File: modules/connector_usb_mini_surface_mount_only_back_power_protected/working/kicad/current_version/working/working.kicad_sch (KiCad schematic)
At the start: 2 parts, among them J3 scumnsmo

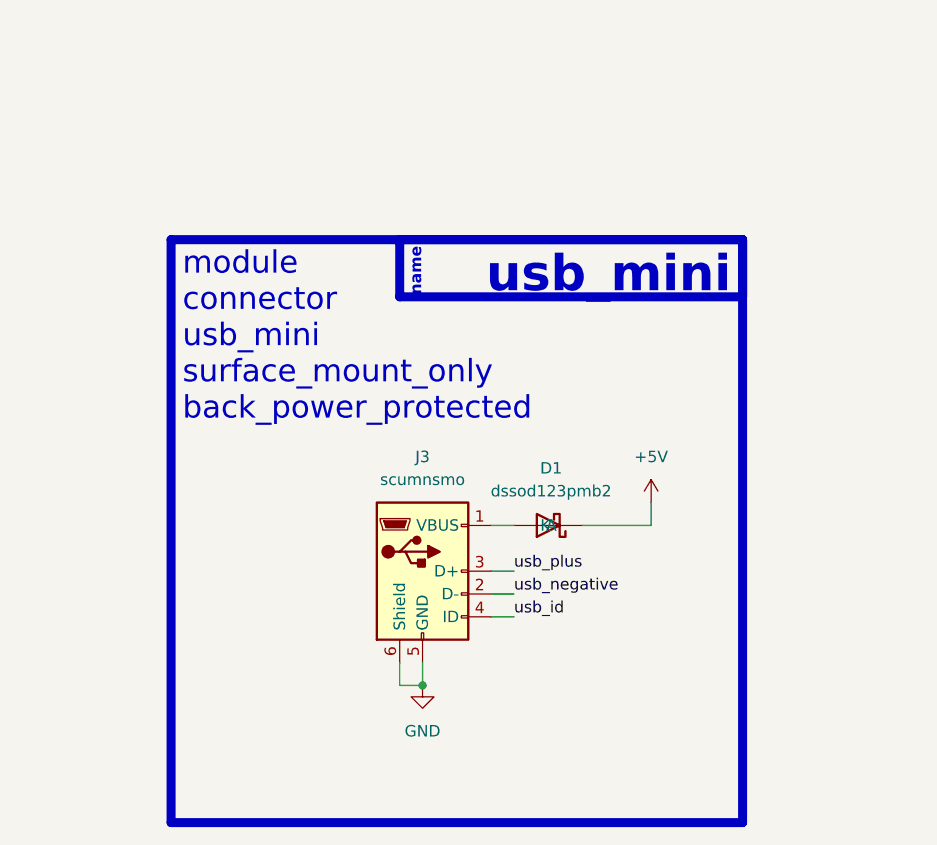
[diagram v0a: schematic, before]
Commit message: a few module workings
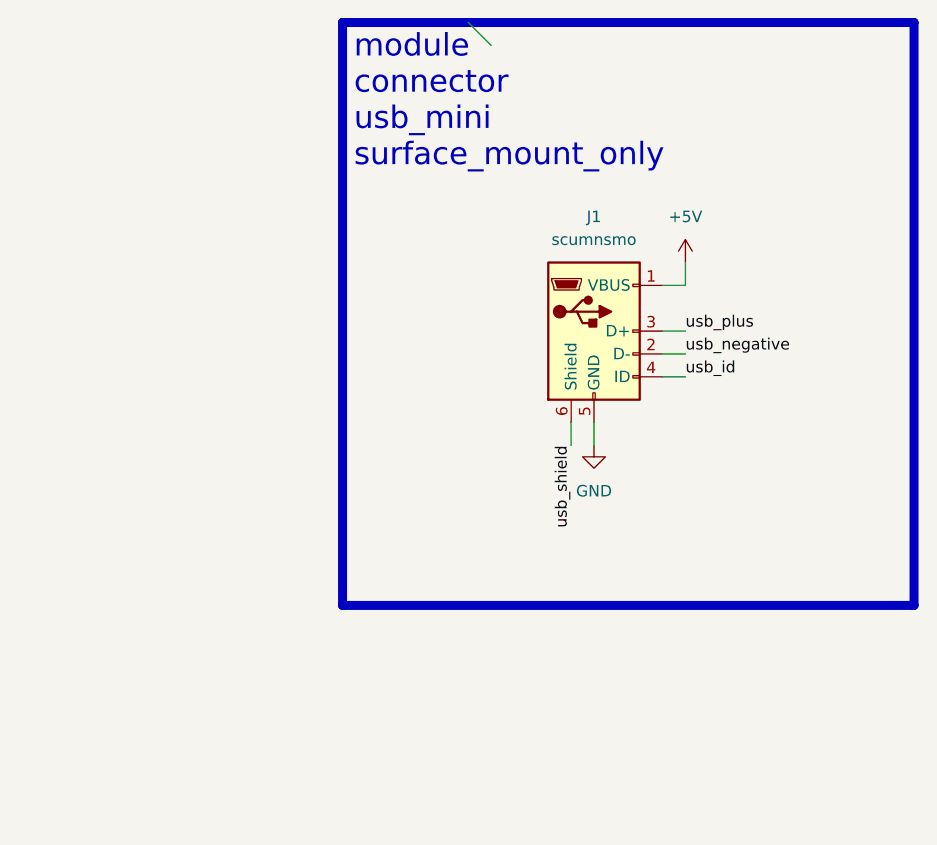
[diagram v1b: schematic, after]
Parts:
- removed D1: dssod123pmb2, oomlout_oomp_part_footprints:dssod123pmb2_electronic_diode_schottky_sod_123_package_marking_b2_mbr0520, symbol oomlout_oomp_part_symbols:dssod123pmb2_electronic_diode_schottky_sod_123_packag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
- removed J3: scumnsmo, oomlout_oomp_part_kicad_footprints:scumnsmo_electronic_socket_usb_mini_surface_mount_only, symbol oomlout_oomp_part_symbols:scumnsmo_electronic_socket_usb_mini_surface_mount_only
- added J1: scumnsmo, scumnsmo_electronic_socket_usb_mini_surface_mount_only, symbol oomlout_oomp_part_symbols:scumnsmo_electronic_socket_usb_mini_surface_mount_only
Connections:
- net +5V: now also J1.1 (VBUS)
- net GND: now also J1.5 (GND)
- net usb_id: now also J1.4 (ID)
- net usb_negative: now also J1.2 (D-)
- net usb_plus: now also J1.3 (D+)
- new net usb_shield: J1.6 (Shield)
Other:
- note added: "module connector usb_mini surface_mount_only"
- note removed: "module connector usb_mini surface_mount_only back_power_protected"
- note removed: "name"
- note removed: "usb_mini"
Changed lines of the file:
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@@
 (kicad_sch (version 20230121) (generator eeschema)
   (paper "A4")
-  (junction (at 146.05 114.3) (diameter 0) (color 0 0 0 0)
-  )
-  (wire (pts (xy 153.67 101.6) (xy 156.21 101.6))
+  (bus_entry (at 151.13 40.64) (size 2.54 2.54)
     (stroke (width 0) (type default))
   )
-  (wire (pts (xy 143.51 114.3) (xy 146.05 114.3))
+  (wire (pts (xy 175.26 69.85) (xy 172.72 69.85))
     (stroke (width 0) (type default))
   )
-  (wire (pts (xy 146.05 111.76) (xy 146.05 114.3))
+  (wire (pts (xy 165.1 85.09) (xy 165.1 87.63))
     (stroke (width 0) (type default))
   )
-  (wire (pts (xy 153.67 96.52) (xy 156.21 96.52))
+  (wire (pts (xy 162.56 85.09) (xy 162.56 87.63))
     (stroke (width 0) (type default))
   )
-  (wire (pts (xy 143.51 111.76) (xy 143.51 114.3))
+  (wire (pts (xy 172.72 74.93) (xy 175.26 74.93))
     (stroke (width 0) (type default))
   )
-  (wire (pts (xy 171.45 96.52) (xy 163.83 96.52))
+  (wire (pts (xy 172.72 80.01) (xy 175.26 80.01))
     (stroke (width 0) (type default))
   )
-  (wire (pts (xy 153.67 104.14) (xy 156.21 104.14))
+  (wire (pts (xy 175.26 67.31) (xy 175.26 69.85))
     (stroke (width 0) (type default))
   )
-  (wire (pts (xy 171.45 93.98) (xy 171.45 96.52))
+  (wire (pts (xy 172.72 77.47) (xy 175.26 77.47))
     (stroke (width 0) (type default))
   )
-  (wire (pts (xy 153.67 106.68) (xy 156.21 106.68))
-    (stroke (width 0) (type default))
-  )
-  (rectangle (start 143.51 64.77) (end 181.61 71.12)
-    (stroke (width 1) (type default))
-    (fill (type color) (color 0 0 0 0))
-  )
-  (rectangle (start 118.11 64.77) (end 181.61 129.54)
+  (rectangle (start 137.16 40.64) (end 200.66 105.41)
     (stroke (width 1) (type default))
     (fill (type none))
   )
-  (text "module\nconnector\nusb_mini\nsurface_mount_only\nback_power_protected\n"
-    (at 119.38 85.09 0)
+  (rectangle (start 199.39 97.79) (end 199.39 97.79)
+    (stroke (width 0) (type default))
+    (fill (type none))
+  )
+  (text "module\nconnector\nusb_mini\nsurface_mount_only\n\n" (at 138.43 60.96 0)
     (effects (font (size 2.5 2.5)) (justify left bottom))
   )
-  (text "usb_mini\n" (at 180.34 71.12 0)
-    (effects (font (size 4 4) (thickness 0.8) bold (color 255 255 255 1)) (justify right bottom))
-  )
-  (text "name" (at 146.05 71.12 90)
-    (effects (font (size 1.27 1.27) (thickness 0.254) bold (color 255 255 255 1)) (justify left bottom))
-  )
-  (label "usb_id" (at 156.21 106.68 0) (fields_autoplaced)
+  (label "usb_id" (at 175.26 80.01 0) (fields_autoplaced)
     (effects (font (size 1.27 1.27)) (justify left bottom))
   )
-  (label "usb_negative" (at 156.21 104.14 0) (fields_autoplaced)
+  (label "usb_plus" (at 175.26 74.93 0) (fields_autoplaced)
     (effects (font (size 1.27 1.27)) (justify left bottom))
   )
-  (label "usb_plus" (at 156.21 101.6 0) (fields_autoplaced)
+  (label "usb_negative" (at 175.26 77.47 0) (fields_autoplaced)
     (effects (font (size 1.27 1.27)) (justify left bottom))
   )
-  (symbol (lib_id "oomlout_oomp_part_symbols:scumnsmo_electronic_socket_usb_mini_surface_mount_only") (at 146.05 101.6 0) (unit 1)
+  (label "usb_shield" (at 162.56 87.63 270) (fields_autoplaced)
+    (effects (font (size 1.27 1.27)) (justify right bottom))
+  )
+  (symbol (lib_id "oomlout_oomp_part_symbols:scumnsmo_electronic_socket_usb_mini_surface_mount_only") (at 165.1 74.93 0) (unit 1)
     (in_bom yes) (on_board yes) (dnp no) (fields_autoplaced)
-    (property "Reference" "J3" (at 146.05 88.9 0)
+    (property "Reference" "J1" (at 165.1 62.23 0)
       (effects (font (size 1.27 1.27)))
     )
-    (property "Value" "scumnsmo" (at 146.05 91.44 0)
+    (property "Value" "scumnsmo" (at 165.1 64.77 0)
       (effects (font (size 1.27 1.27)))
     )
-    (property "Footprint" "oomlout_oomp_part_kicad_footprints:scumnsmo_electronic_socket_usb_mini_surface_mount_only" (at 149.86 102.87 0)
+    (property "Footprint" "scumnsmo_electronic_socket_usb_mini_surface_mount_only" (at 168.91 76.2 0)
       (effects (font (size 1.27 1.27)) hide)
     )
-    (property "Datasheet" "https://github.com/oomlout/oomlout_oomp_v3/parts/electronic_socket_usb_mini_surface_mount_only/datasheet.pdf" (at 149.86 102.87 0)
+    (property "Datasheet" "https://github.com/oomlout/oomlout_oomp_v3/parts/electronic_socket_usb_mini_surface_mount_only/datasheet.pdf" (at 168.91 76.2 0)
       (effects (font (size 1.27 1.27)) hide)
     )
@@
     (instances
       (project "working"
-        (path "/5407c114-4107-4d84-8382-1717fb9d687c"
-          (reference "J3") (unit 1)
-        )
-      )
-      (project "working"
         (path "/d7ac9d55-1973-40f4-b2a5-38a433b49fa0"
           (reference "J1") (unit 1)
@@
     )
   )
-  (symbol (lib_id "oomlout_oomp_part_symbols:dssod123pmb2_electronic_diode_schottky_sod_123_package_marking_b2_mbr0520") (at 160.02 96.52 180) (unit 1)
+  (symbol (lib_id "power:+5V") (at 175.26 67.31 0) (unit 1)
     (in_bom yes) (on_board yes) (dnp no) (fields_autoplaced)
-    (property "Reference" "D1" (at 160.3375 90.17 0)
+    (property "Reference" "#PWR04" (at 175.26 71.12 0)
+      (effects (font (size 1.27 1.27)) hide)
+    )
+    (property "Value" "+5V" (at 175.26 62.23 0)
       (effects (font (size 1.27 1.27)))
     )
-    (property "Value" "dssod123pmb2" (at 160.3375 92.71 0)
-      (effects (font (size 1.27 1.27)))
-    )
-    (property "Footprint" "oomlout_oomp_part_footprints:dssod123pmb2_electronic_diode_schottky_sod_123_package_marking_b2_mbr0520" (at 160.02 96.52 0)
+    (property "Footprint" "" (at 175.26 67.31 0)
       (effects (font (size 1.27 1.27)) hide)
     )
-    (property "Datasheet" "https://github.com/oomlout/oomlout_oomp_v3/parts/electronic_diode_schottky_sod_123_package_marking_b2_mbr0520/datasheet.pdf" (at 160.02 96.52 0)
-      (effects (font (size 1.27 1.27)) hide)
-    )
-    (pin "1")
-    (pin "2")
-    (instances
-      (project "working"
-        (path "/d7ac9d55-1973-40f4-b2a5-38a433b49fa0"
-          (reference "D1") (unit 1)
-        )
-      )
-    )
-  )
-  (symbol (lib_id "power:+5V") (at 171.45 93.98 0) (unit 1)
-    (in_bom yes) (on_board yes) (dnp no) (fields_autoplaced)
-    (property "Reference" "#PWR013" (at 171.45 97.79 0)
-      (effects (font (size 1.27 1.27)) hide)
-    )
-    (property "Value" "+5V" (at 171.45 88.9 0)
-      (effects (font (size 1.27 1.27)))
-    )
-    (property "Footprint" "" (at 171.45 93.98 0)
-      (effects (font (size 1.27 1.27)) hide)
-    )
-    (property "Datasheet" "" (at 171.45 93.98 0)
+    (property "Datasheet" "" (at 175.26 67.31 0)
       (effects (font (size 1.27 1.27)) hide)
     )
@@
     (instances
       (project "working"
-        (path "/5407c114-4107-4d84-8382-1717fb9d687c"
-          (reference "#PWR013") (unit 1)
-        )
-      )
-      (project "working"
         (path "/d7ac9d55-1973-40f4-b2a5-38a433b49fa0"
-          (reference "#PWR02") (unit 1)
+          (reference "#PWR04") (unit 1)
         )
       )
     )
   )
-  (symbol (lib_id "power:GND") (at 146.05 114.3 0) (unit 1)
+  (symbol (lib_id "power:GND") (at 165.1 87.63 0) (unit 1)
     (in_bom yes) (on_board yes) (dnp no) (fields_autoplaced)
-    (property "Reference" "#PWR012" (at 146.05 120.65 0)
+    (property "Reference" "#PWR03" (at 165.1 93.98 0)
       (effects (font (size 1.27 1.27)) hide)
     )
-    (property "Value" "GND" (at 146.05 119.38 0)
+    (property "Value" "GND" (at 165.1 92.71 0)
       (effects (font (size 1.27 1.27)))
     )
-    (property "Footprint" "" (at 146.05 114.3 0)
+    (property "Footprint" "" (at 165.1 87.63 0)
       (effects (font (size 1.27 1.27)) hide)
     )
-    (property "Datasheet" "" (at 146.05 114.3 0)
+    (property "Datasheet" "" (at 165.1 87.63 0)
       (effects (font (size 1.27 1.27)) hide)
     )
@@
     (instances
       (project "working"
-        (path "/5407c114-4107-4d84-8382-1717fb9d687c"
-          (reference "#PWR012") (unit 1)
+        (path "/d7ac9d55-1973-40f4-b2a5-38a433b49fa0"
+          (reference "#PWR03") (unit 1)
         )
       )
-      (project "working"
-        (path "/d7ac9d55-1973-40f4-b2a5-38a433b49fa0"
-          (reference "#PWR01") (unit 1)
-        )
-      )
